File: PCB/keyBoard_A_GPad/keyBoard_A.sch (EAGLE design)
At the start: 528 parts, among them IC1 74HC04N, IC2 LMV358IDGKR, J1 J, J10 J, J11 J, J12 J, J13 J, J14 J, J15 J, J16 J, J17 J, J18 J, J19 J, J2 J, J20 J, J21 J, J22 J, J23 J, J24 J, J25 J, J26 J, J27 J, J28 J, J29 J, J3 J, J30 J, J31 J, J32 J, J33 J, J34 J, J35 J, J36 J, J37 J, J38 J, J39 J, J4 J, J40 J, J41 J, J42 J, J43 J, J44 J, J45 J, J46 J, J47 USB MICRO, J48 J, J49 J, J5 J, J50 J, J51 J, J52 J, J53 J, J54 J, J55 J, J56 J, J57 J, J58 J, J59 J, J6 J, J60 J, J61 J, J62 J, J63 J, J64 J, J65 J, J66 J, J67 J, J68 J, J69 J, J7 J, J70 J, J71 J, J72 J, J73 J, J74 J, J75 J, J76 J, J77 J, J78 J, J79 J, J8 J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

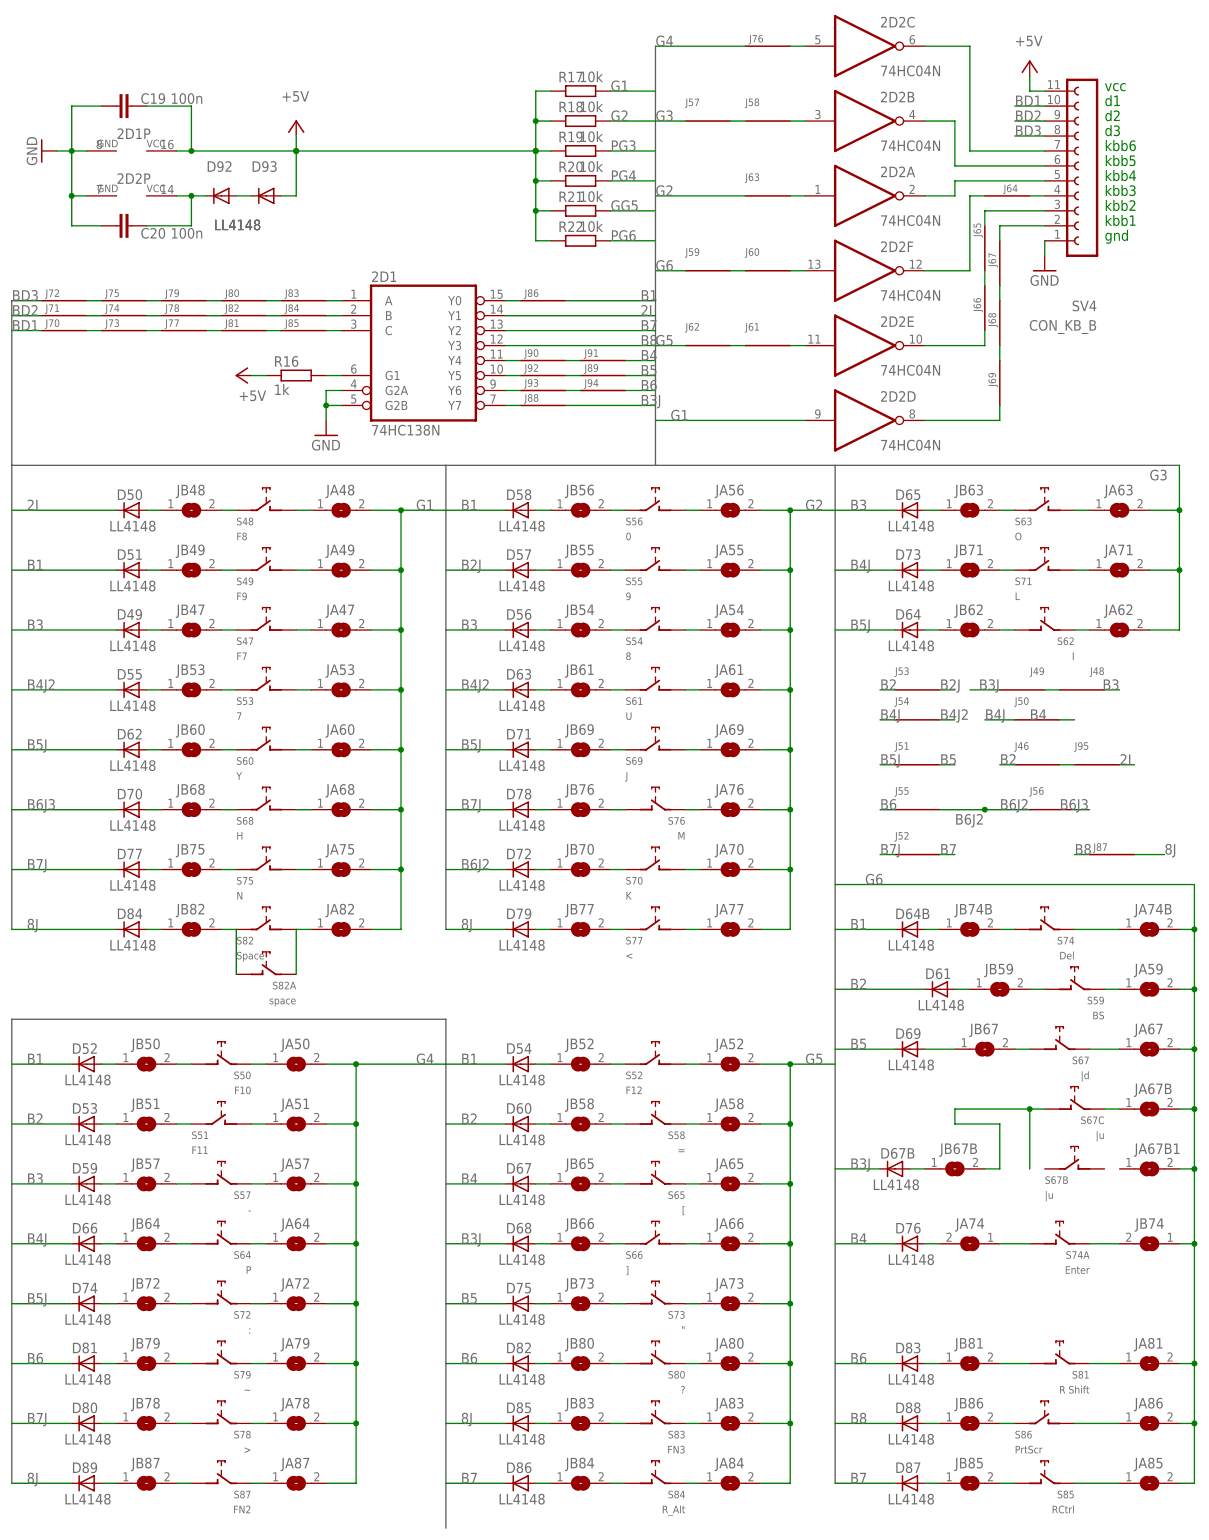
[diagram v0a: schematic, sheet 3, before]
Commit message: pcb b > ab .2
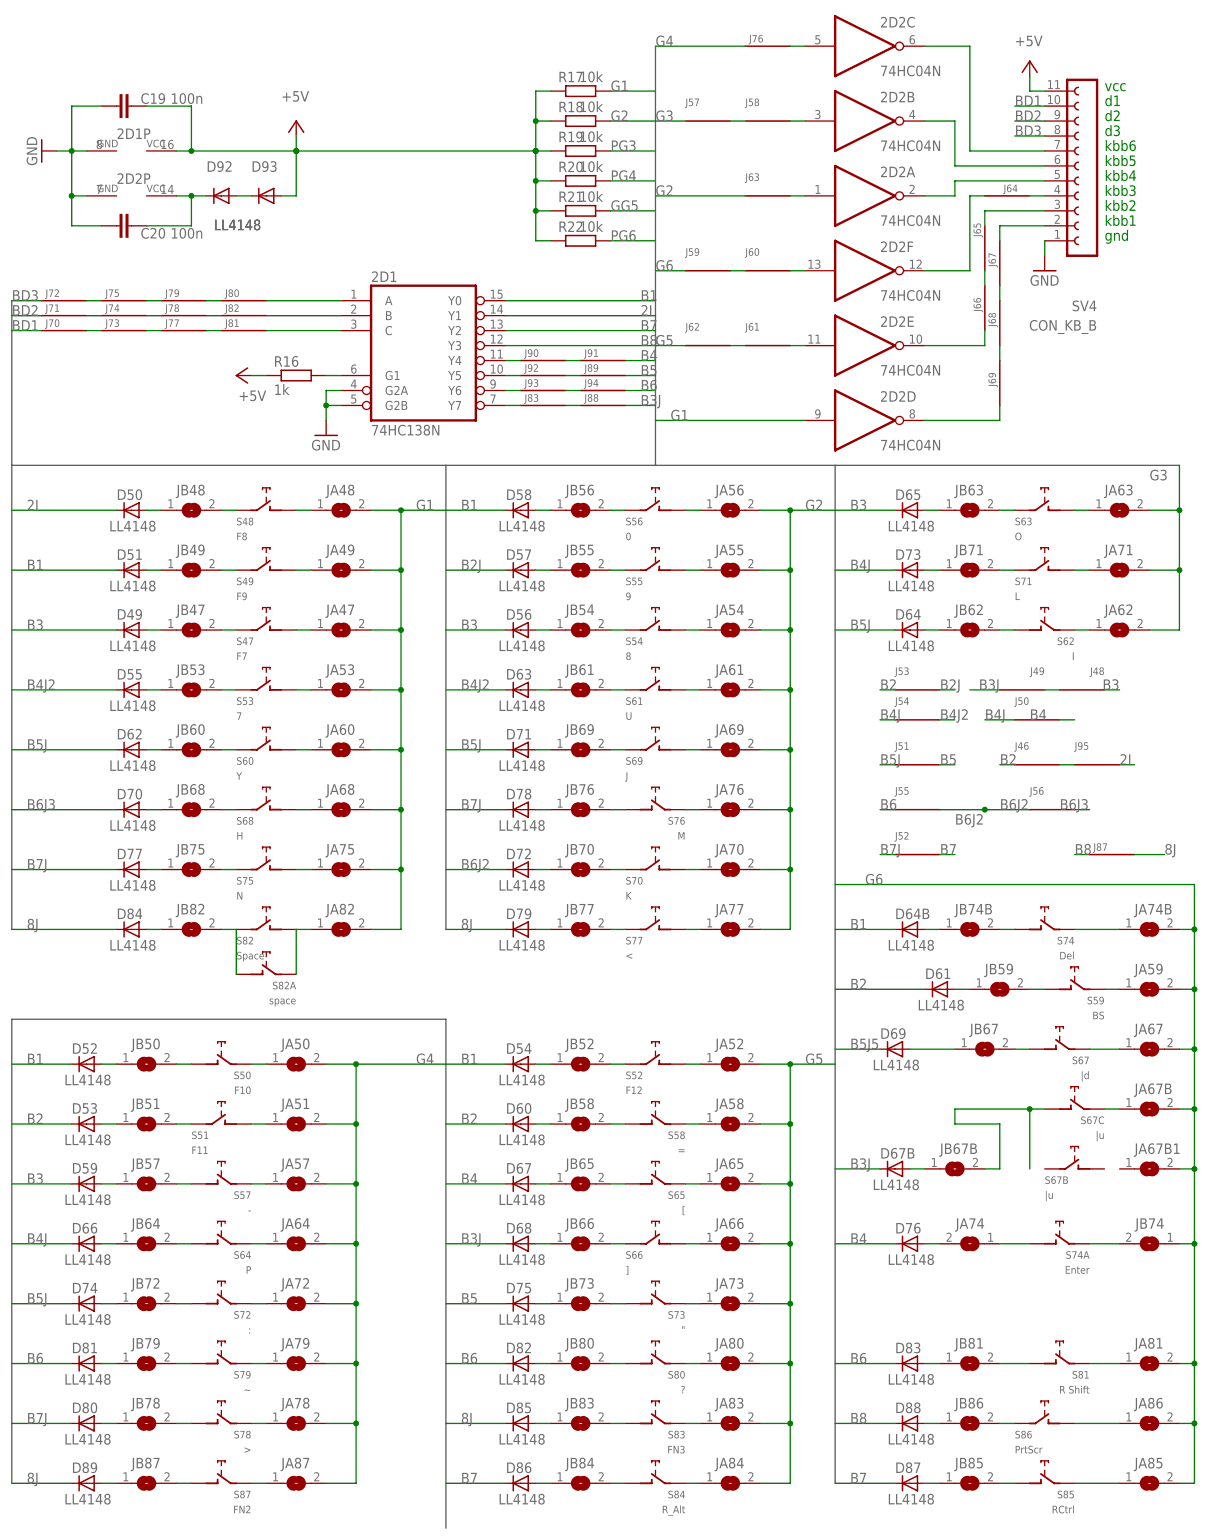
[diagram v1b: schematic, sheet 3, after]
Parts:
- removed J84, J85, J86: J, detali2:J
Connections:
- net N$401 renamed B5J4
- removed net N$392: 2D1A.A, J83.P$1
- removed net N$393: 2D1A.B, J84.P$1
- removed net N$394: 2D1A.C, J85.P$1
- removed net N$395: 2D1A.Y0, J86.P$2
- removed net N$398: 2D1A.Y7, J88.P$2
- removed net N$404: 2D1A.Y5, J92.P$2
- new net B5J5: 2D1A.Y5, D69.C, J92.P$2
- new net N$117: 2D1A.Y7, J83.P$2
- new net N$197: J83.P$1, J88.P$2
- net B1: now also 2D1A.Y0; no longer J86.P$1
- net B5: no longer D69.C
- net N$388: now also 2D1A.A; no longer J83.P$2
- net N$389: now also 2D1A.B; no longer J84.P$2
- net N$391: now also 2D1A.C; no longer J85.P$2
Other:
- moved on the sheet: D69, J83, J88
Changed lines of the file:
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@@
 <part name="J81" library="detali2" deviceset="J" device="" value=""/>
 <part name="J82" library="detali2" deviceset="J" device="" value=""/>
-<part name="J83" library="detali2" deviceset="J" device="" value=""/>
-<part name="J84" library="detali2" deviceset="J" device="" value=""/>
-<part name="J85" library="detali2" deviceset="J" device="" value=""/>
-<part name="J86" library="detali2" deviceset="J" device="" value=""/>
 <part name="J87" library="detali2" deviceset="J" device="" value=""/>
 <part name="J88" library="detali2" deviceset="J" device="" value=""/>
@@
 <part name="S44A" library="cherrymx" deviceset="CHERRY-MX" device="" value="Fn1"/>
 <part name="S82A" library="cherrymx" deviceset="CHERRY-MX" device="" value="space"/>
+<part name="J83" library="detali2" deviceset="J" device="" value=""/>
 </parts>
 <sheets>
@@
 <instance part="D67" gate="G$1" x="96.52" y="60.96"/>
 <instance part="D68" gate="G$1" x="96.52" y="50.8"/>
-<instance part="D69" gate="G$1" x="162.56" y="83.82"/>
+<instance part="D69" gate="G$1" x="160.02" y="83.82"/>
 <instance part="D70" gate="G$1" x="30.48" y="124.46"/>
 <instance part="D71" gate="G$1" x="96.52" y="134.62"/>
@@
 <attribute name="NAME" x="46.355" y="208.915" size="1.27" layer="95"/>
 </instance>
-<instance part="J83" gate="G$1" x="58.42" y="210.82" smashed="yes">
-<attribute name="NAME" x="56.515" y="211.455" size="1.27" layer="95"/>
-</instance>
-<instance part="J84" gate="G$1" x="58.42" y="208.28" smashed="yes">
-<attribute name="NAME" x="56.515" y="208.915" size="1.27" layer="95"/>
-</instance>
-<instance part="J85" gate="G$1" x="58.42" y="205.74" smashed="yes">
-<attribute name="NAME" x="56.515" y="206.375" size="1.27" layer="95"/>
-</instance>
-<instance part="J86" gate="G$1" x="99.06" y="210.82" smashed="yes">
-<attribute name="NAME" x="97.155" y="211.455" size="1.27" layer="95"/>
-</instance>
 <instance part="J87" gate="G$1" x="195.58" y="116.84" smashed="yes">
 <attribute name="NAME" x="193.675" y="117.475" size="1.27" layer="95"/>
 </instance>
-<instance part="J88" gate="G$1" x="99.06" y="193.04" smashed="yes">
-<attribute name="NAME" x="97.155" y="193.675" size="1.27" layer="95"/>
+<instance part="J88" gate="G$1" x="109.22" y="193.04" smashed="yes">
+<attribute name="NAME" x="107.315" y="193.675" size="1.27" layer="95"/>
 </instance>
 <instance part="J89" gate="G$1" x="109.22" y="198.12" smashed="yes">
@@
 </instance>
 <instance part="S82A" gate="G$1" x="53.34" y="96.52" rot="MR0"/>
+<instance part="J83" gate="G$1" x="99.06" y="193.04" smashed="yes">
+<attribute name="NAME" x="97.155" y="193.675" size="1.27" layer="95"/>
+</instance>
 </instances>
 <busses>
@@
 <pinref part="JB67" gate="1" pin="1"/>
 <pinref part="D69" gate="G$1" pin="A"/>
-<wire x1="165.1" y1="83.82" x2="170.18" y2="83.82" width="0.1524" layer="91"/>
+<wire x1="162.56" y1="83.82" x2="170.18" y2="83.82" width="0.1524" layer="91"/>
 </segment>
 </net>
@@
 </segment>
 <segment>
-<pinref part="J86" gate="G$1" pin="P$1"/>
-<wire x1="104.14" y1="210.82" x2="119.38" y2="210.82" width="0.1524" layer="91"/>
 <label x="116.84" y="210.82" size="1.778" layer="95"/>
+<pinref part="2D1" gate="A" pin="Y0"/>
+<wire x1="93.98" y1="210.82" x2="119.38" y2="210.82" width="0.1524" layer="91"/>
 </segment>
 </net>
@@
 <net name="B5" class="0">
 <segment>
-<pinref part="D69" gate="G$1" pin="C"/>
-<wire x1="149.86" y1="83.82" x2="160.02" y2="83.82" width="0.1524" layer="91"/>
-<label x="152.4" y="83.82" size="1.778" layer="95"/>
-</segment>
-<segment>
 <pinref part="D75" gate="G$1" pin="C"/>
 <wire x1="83.82" y1="40.64" x2="93.98" y2="40.64" width="0.1524" layer="91"/>
@@
 <segment>
 <pinref part="J80" gate="G$1" pin="P$1"/>
-<pinref part="J83" gate="G$1" pin="P$2"/>
-<wire x1="53.34" y1="210.82" x2="55.88" y2="210.82" width="0.1524" layer="91"/>
+<pinref part="2D1" gate="A" pin="A"/>
+<wire x1="53.34" y1="210.82" x2="66.04" y2="210.82" width="0.1524" layer="91"/>
 </segment>
 </net>
@@
 <segment>
 <pinref part="J82" gate="G$1" pin="P$1"/>
-<pinref part="J84" gate="G$1" pin="P$2"/>
-<wire x1="53.34" y1="208.28" x2="55.88" y2="208.28" width="0.1524" layer="91"/>
+<pinref part="2D1" gate="A" pin="B"/>
+<wire x1="53.34" y1="208.28" x2="66.04" y2="208.28" width="0.1524" layer="91"/>
 </segment>
 </net>
@@
 <segment>
 <pinref part="J81" gate="G$1" pin="P$1"/>
-<pinref part="J85" gate="G$1" pin="P$2"/>
-<wire x1="53.34" y1="205.74" x2="55.88" y2="205.74" width="0.1524" layer="91"/>
-</segment>
-</net>
-<net name="N$392" class="0">
-<segment>
-<pinref part="J83" gate="G$1" pin="P$1"/>
-<pinref part="2D1" gate="A" pin="A"/>
-<wire x1="63.5" y1="210.82" x2="66.04" y2="210.82" width="0.1524" layer="91"/>
-</segment>
-</net>
-<net name="N$393" class="0">
-<segment>
-<pinref part="J84" gate="G$1" pin="P$1"/>
-<pinref part="2D1" gate="A" pin="B"/>
-<wire x1="63.5" y1="208.28" x2="66.04" y2="208.28" width="0.1524" layer="91"/>
-</segment>
-</net>
-<net name="N$394" class="0">
-<segment>
-<pinref part="J85" gate="G$1" pin="P$1"/>
 <pinref part="2D1" gate="A" pin="C"/>
-<wire x1="63.5" y1="205.74" x2="66.04" y2="205.74" width="0.1524" layer="91"/>
-</segment>
-</net>
-<net name="N$395" class="0">
-<segment>
-<pinref part="2D1" gate="A" pin="Y0"/>
-<pinref part="J86" gate="G$1" pin="P$2"/>
-<wire x1="93.98" y1="210.82" x2="96.52" y2="210.82" width="0.1524" layer="91"/>
+<wire x1="53.34" y1="205.74" x2="66.04" y2="205.74" width="0.1524" layer="91"/>
 </segment>
 </net>
@@
 </segment>
 </net>
-<net name="N$398" class="0">
-<segment>
-<pinref part="2D1" gate="A" pin="Y7"/>
-<pinref part="J88" gate="G$1" pin="P$2"/>
-<wire x1="93.98" y1="193.04" x2="96.52" y2="193.04" width="0.1524" layer="91"/>
-</segment>
-</net>
 <net name="N$399" class="0">
 <segment>
@@
 </segment>
 </net>
-<net name="N$401" class="0">
+<net name="B5J4" class="0">
 <segment>
 <pinref part="J92" gate="G$1" pin="P$1"/>
@@
 </segment>
 </net>
-<net name="N$404" class="0">
+<net name="B5J5" class="0">
 <segment>
 <pinref part="J92" gate="G$1" pin="P$2"/>
@@
 <wire x1="96.52" y1="198.12" x2="93.98" y2="198.12" width="0.1524" layer="91"/>
 </segment>
+<segment>
+<pinref part="D69" gate="G$1" pin="C"/>
+<wire x1="149.86" y1="83.82" x2="157.48" y2="83.82" width="0.1524" layer="91"/>
+<label x="152.4" y="83.82" size="1.778" layer="95"/>
+</segment>
 </net>
 <net name="N$405" class="0">
@@
 <segment>
 <pinref part="J88" gate="G$1" pin="P$1"/>
-<wire x1="104.14" y1="193.04" x2="119.38" y2="193.04" width="0.1524" layer="91"/>
+<wire x1="114.3" y1="193.04" x2="119.38" y2="193.04" width="0.1524" layer="91"/>
 <label x="116.84" y="193.04" size="1.778" layer="95"/>
 </segment>
 </net>
+<net name="N$117" class="0">
+<segment>
+<pinref part="2D1" gate="A" pin="Y7"/>
+<pinref part="J83" gate="G$1" pin="P$2"/>
+<wire x1="93.98" y1="193.04" x2="96.52" y2="193.04" width="0.1524" layer="91"/>
+</segment>
+</net>
+<net name="N$197" class="0">
+<segment>
+<pinref part="J83" gate="G$1" pin="P$1"/>
+<pinref part="J88" gate="G$1" pin="P$2"/>
+<wire x1="104.14" y1="193.04" x2="106.68" y2="193.04" width="0.1524" layer="91"/>
+</segment>
+</net>
